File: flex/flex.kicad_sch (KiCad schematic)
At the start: 143 parts, among them J1 NA_Conn_01x06_Female, J2 NA_Conn_01x05_Female, J3 NA_Conn_01x06_Female, J4 NA_Conn_01x03_Female, J5 NA_Conn_01x03_Female, SW1 SW_Push, SW10 SW_Push, SW11 SW_Push, SW12 SW_Push, SW13 SW_Push, SW14 SW_Push, SW15 SW_Push, SW16 SW_Push, SW17 SW_Push, SW18 SW_Push, SW19 SW_Push, SW2 SW_Push, SW20 SW_Push, SW21 SW_Push, SW22 SW_Push, SW23 SW_Push, SW24 SW_Push, SW3 SW_Push, SW4 SW_Push, SW5 SW_Push, SW6 SW_Push, SW7 SW_Push, SW8 SW_Push, SW9 SW_Push

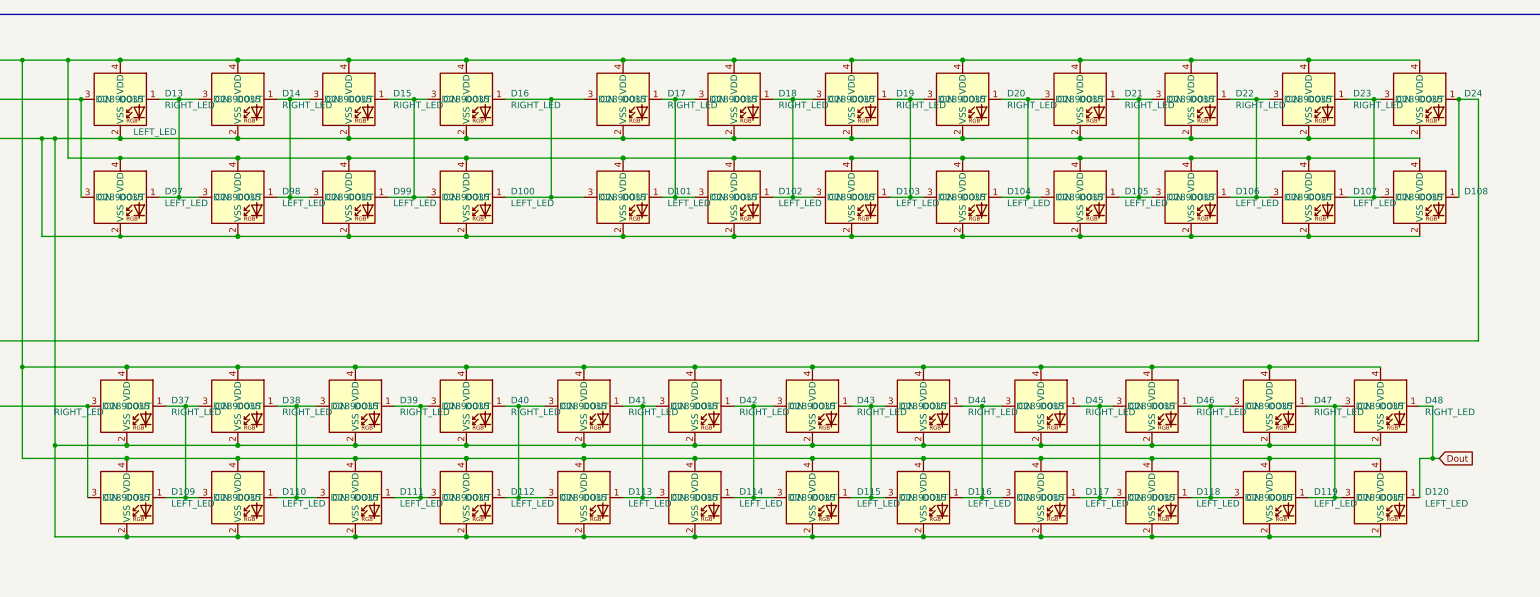
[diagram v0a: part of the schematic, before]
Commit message: BOM
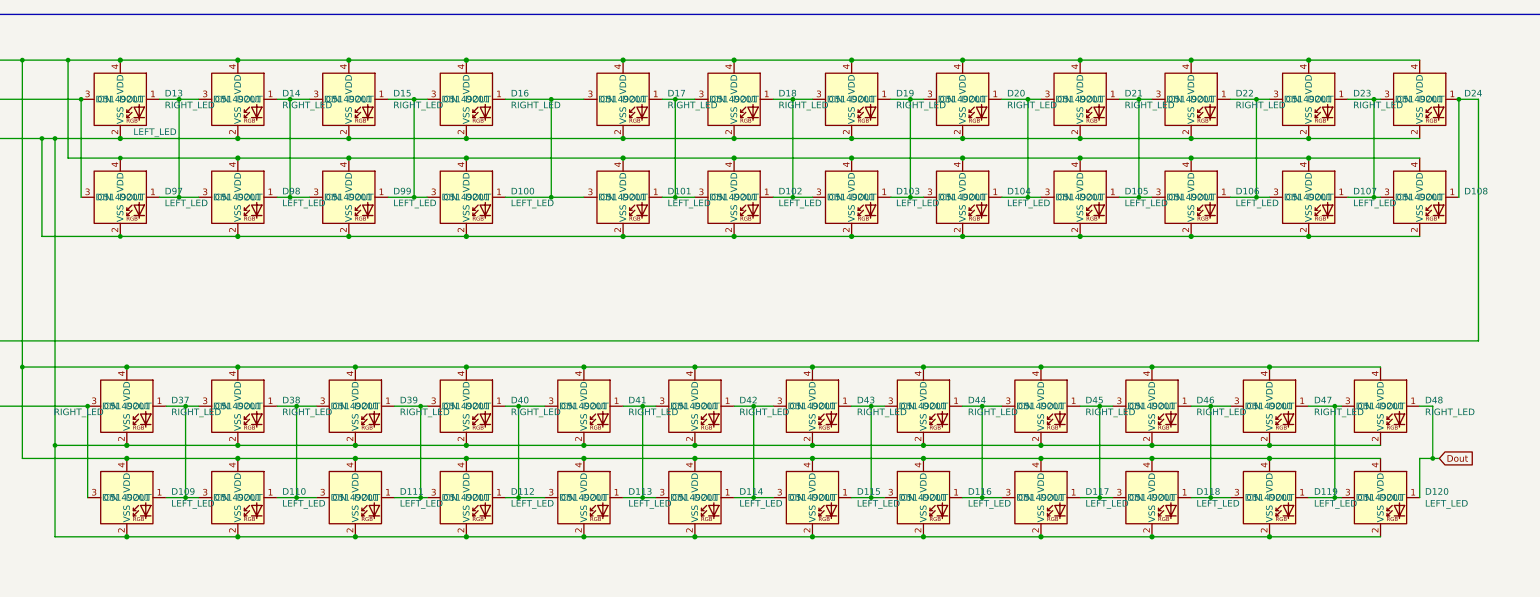
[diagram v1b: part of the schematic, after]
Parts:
- D100, D101, D102, D103, D104, D105, D106, D107, D108, D109, D110, D111, D112, D113, D114, D115, D116, D117, D118, D119, D120, D13, D14, D15, D16, D17, D18, D19, D20, D21, D22, D23, D24, D37, D38, D39, D40, D41, D42, D43, D44, D45, D46, D47, D48, D97, D98, D99: LCSC C2890035 -> C5149201
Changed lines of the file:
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@@
 			)
 		)
-		(property "LCSC" "C2890035"
+		(property "LCSC" "C5149201"
 			(at 148.59 204.47 0)
 			(effects
@@
 			)
 		)
-		(property "LCSC" "C2890035"
+		(property "LCSC" "C5149201"
 			(at 193.04 204.47 0)
 			(effects
@@
 			)
 		)
-		(property "LCSC" "C2890035"
+		(property "LCSC" "C5149201"
 			(at 267.97 127 0)
 			(effects
@@
 			)
 		)
-		(property "LCSC" "C2890035"
+		(property "LCSC" "C5149201"
 			(at 148.59 186.69 0)
 			(effects
@@
 			)
 		)
-		(property "LCSC" "C2890035"
+		(property "LCSC" "C5149201"
 			(at 81.28 127 0)
 			(effects
@@
 			)
 		)
-		(property "LCSC" "C2890035"
+		(property "LCSC" "C5149201"
 			(at 312.42 127 0)
 			(effects
@@
 			)
 		)
-		(property "LCSC" "C2890035"
+		(property "LCSC" "C5149201"
 			(at 289.56 146.05 0)
 			(effects
@@
 			)
 		)
-		(property "LCSC" "C2890035"
+		(property "LCSC" "C5149201"
 			(at 223.52 127 0)
 			(effects
@@
 			)
 		)
-		(property "LCSC" "C2890035"
+		(property "LCSC" "C5149201"
 			(at 82.55 186.69 0)
 			(effects
@@
 			)
 		)
-		(property "LCSC" "C2890035"
+		(property "LCSC" "C5149201"
 			(at 104.14 186.69 0)
 			(effects
@@
 			)
 		)
-		(property "LCSC" "C2890035"
+		(property "LCSC" "C5149201"
 			(at 289.56 127 0)
 			(effects
@@
 			)
 		)
-		(property "LCSC" "C2890035"
+		(property "LCSC" "C5149201"
 			(at 312.42 146.05 0)
 			(effects
@@
 			)
 		)
-		(property "LCSC" "C2890035"
+		(property "LCSC" "C5149201"
 			(at 127 186.69 0)
 			(effects
@@
 			)
 		)
-		(property "LCSC" "C2890035"
+		(property "LCSC" "C5149201"
 			(at 193.04 186.69 0)
 			(effects
@@
 			)
 		)
-		(property "LCSC" "C2890035"
+		(property "LCSC" "C5149201"
 			(at 245.11 146.05 0)
 			(effects
@@
 			)
 		)
-		(property "LCSC" "C2890035"
+		(property "LCSC" "C5149201"
 			(at 127 204.47 0)
 			(effects
@@
 			)
 		)
-		(property "LCSC" "C2890035"
+		(property "LCSC" "C5149201"
 			(at 81.28 146.05 0)
 			(effects
@@
 			)
 		)
-		(property "LCSC" "C2890035"
+		(property "LCSC" "C5149201"
 			(at 326.39 186.69 0)
 			(effects
@@
 			)
 		)
-		(property "LCSC" "C2890035"
+		(property "LCSC" "C5149201"
 			(at 334.01 146.05 0)
 			(effects
@@
 			)
 		)
-		(property "LCSC" "C2890035"
+		(property "LCSC" "C5149201"
 			(at 281.94 204.47 0)
 			(effects
@@
 			)
 		)
-		(property "LCSC" "C2890035"
+		(property "LCSC" "C5149201"
 			(at 104.14 146.05 0)
 			(effects
@@
 			)
 		)
-		(property "LCSC" "C2890035"
+		(property "LCSC" "C5149201"
 			(at 179.07 127 0)
 			(effects
@@
 			)
 		)
-		(property "LCSC" "C2890035"
+		(property "LCSC" "C5149201"
 			(at 215.9 204.47 0)
 			(effects
@@
 			)
 		)
-		(property "LCSC" "C2890035"
+		(property "LCSC" "C5149201"
 			(at 200.66 127 0)
 			(effects
@@
 			)
 		)
-		(property "LCSC" "C2890035"
+		(property "LCSC" "C5149201"
 			(at 223.52 146.05 0)
 			(effects
@@
 			)
 		)
-		(property "LCSC" "C2890035"
+		(property "LCSC" "C5149201"
 			(at 200.66 146.05 0)
 			(effects
@@
 			)
 		)
-		(property "LCSC" "C2890035"
+		(property "LCSC" "C5149201"
 			(at 260.35 186.69 0)
 			(effects
@@
 			)
 		)
-		(property "LCSC" "C2890035"
+		(property "LCSC" "C5149201"
 			(at 304.8 186.69 0)
 			(effects
@@
 			)
 		)
-		(property "LCSC" "C2890035"
+		(property "LCSC" "C5149201"
 			(at 260.35 204.47 0)
 			(effects
@@
 			)
 		)
-		(property "LCSC" "C2890035"
+		(property "LCSC" "C5149201"
 			(at 237.49 204.47 0)
 			(effects
@@
 			)
 		)
-		(property "LCSC" "C2890035"
+		(property "LCSC" "C5149201"
 			(at 334.01 127 0)
 			(effects
@@
 			)
 		)
-		(property "LCSC" "C2890035"
+		(property "LCSC" "C5149201"
 			(at 171.45 204.47 0)
 			(effects
@@
 			)
 		)
-		(property "LCSC" "C2890035"
+		(property "LCSC" "C5149201"
 			(at 104.14 204.47 0)
 			(effects
@@
 			)
 		)
-		(property "LCSC" "C2890035"
+		(property "LCSC" "C5149201"
 			(at 215.9 186.69 0)
 			(effects
@@
 			)
 		)
-		(property "LCSC" "C2890035"
+		(property "LCSC" "C5149201"
 			(at 82.55 204.47 0)
 			(effects
@@
 			)
 		)
-		(property "LCSC" "C2890035"
+		(property "LCSC" "C5149201"
 			(at 179.07 146.05 0)
 			(effects
@@
 			)
 		)
-		(property "LCSC" "C2890035"
+		(property "LCSC" "C5149201"
 			(at 171.45 186.69 0)
 			(effects
@@
 			)
 		)
-		(property "LCSC" "C2890035"
+		(property "LCSC" "C5149201"
 			(at 125.73 127 0)
 			(effects
@@
 			)
 		)
-		(property "LCSC" "C2890035"
+		(property "LCSC" "C5149201"
 			(at 326.39 204.47 0)
 			(effects
@@
 			)
 		)
-		(property "LCSC" "C2890035"
+		(property "LCSC" "C5149201"
 			(at 148.59 127 0)
 			(effects
@@
 			)
 		)
-		(property "LCSC" "C2890035"
+		(property "LCSC" "C5149201"
 			(at 304.8 204.47 0)
 			(effects
@@
 			)
 		)
-		(property "LCSC" "C2890035"
+		(property "LCSC" "C5149201"
 			(at 245.11 127 0)
 			(effects
@@
 			)
 		)
-		(property "LCSC" "C2890035"
+		(property "LCSC" "C5149201"
 			(at 104.14 127 0)
 			(effects
@@
 			)
 		)
-		(property "LCSC" "C2890035"
+		(property "LCSC" "C5149201"
 			(at 281.94 186.69 0)
 			(effects
@@
 			)
 		)
-		(property "LCSC" "C2890035"
+		(property "LCSC" "C5149201"
 			(at 237.49 186.69 0)
 			(effects
@@
 			)
 		)
-		(property "LCSC" "C2890035"
+		(property "LCSC" "C5149201"
 			(at 125.73 146.05 0)
 			(effects
@@
 			)
 		)
-		(property "LCSC" "C2890035"
+		(property "LCSC" "C5149201"
 			(at 267.97 146.05 0)
 			(effects
@@
 			)
 		)
-		(property "LCSC" "C2890035"
+		(property "LCSC" "C5149201"
 			(at 148.59 146.05 0)
 			(effects
